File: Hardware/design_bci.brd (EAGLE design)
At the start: 100 x 80 mm, 10 parts, among them IC1 AD623N

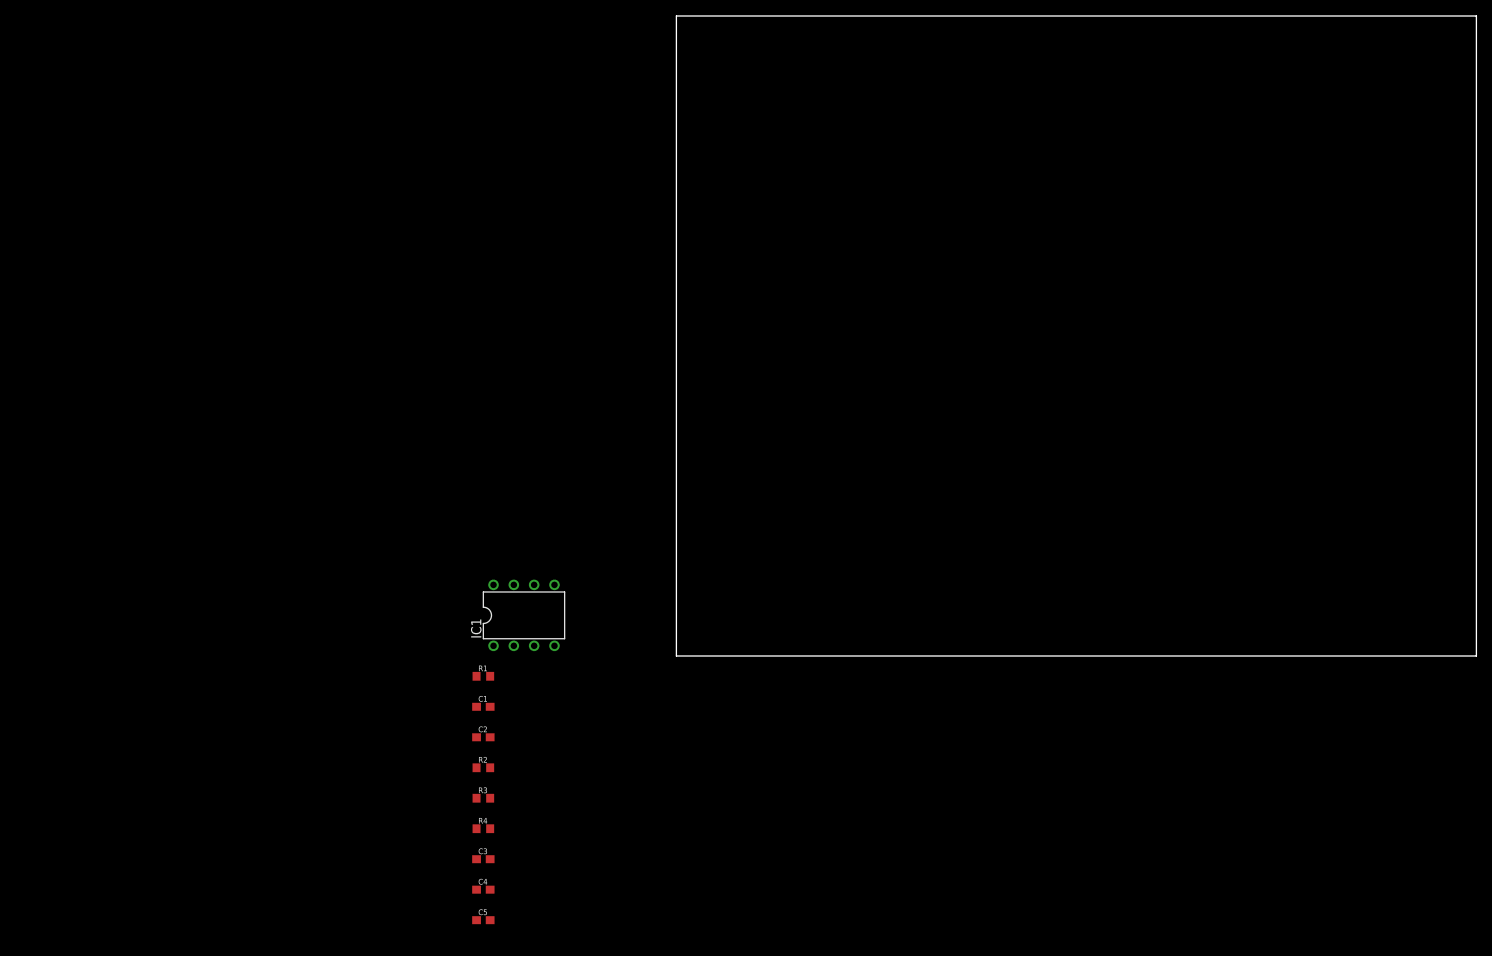
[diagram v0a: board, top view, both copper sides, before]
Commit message: updated
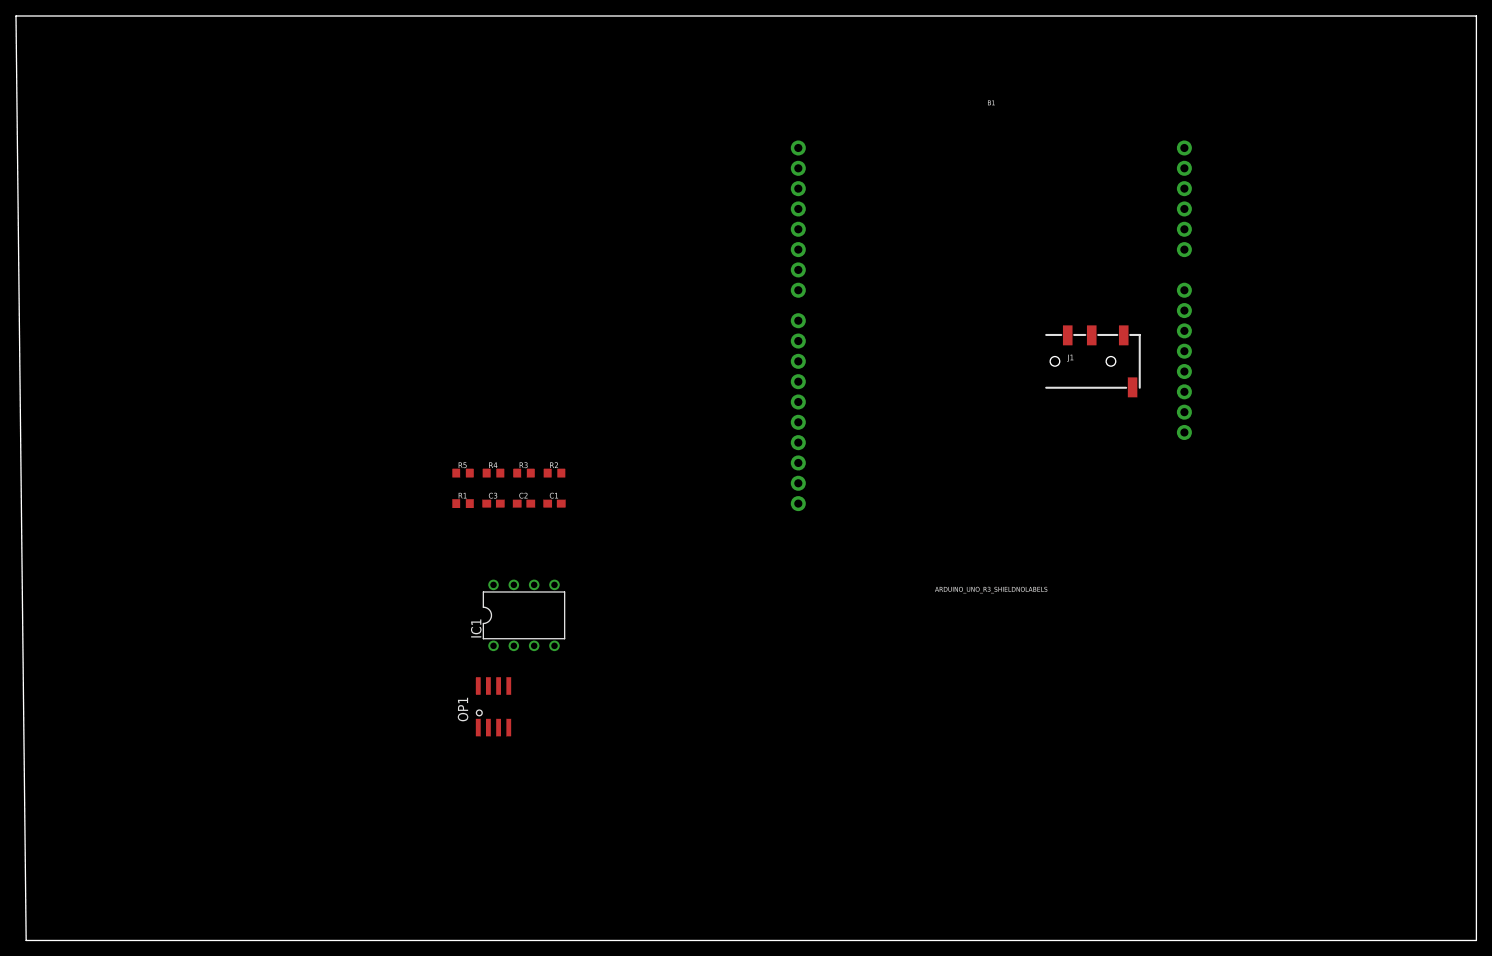
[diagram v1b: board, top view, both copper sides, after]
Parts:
- removed C4, C5: (no value), LinnesLab-Passives:C0603
- added B1: ARDUINO_UNO_R3_SHIELDNOLABELS, LinnesLab-Microcontrollers:UNO_R3_SHIELD_NOLABELS
- added J1: (no value), LinnesLab-Connectors:AUDIO_JACK_3.5MM_TRRS_SMD_RA
- added OP1: (no value), LinnesLab-AnalogIC:SO8
- added R5: (no value), LinnesLab-Passives:R0603
- moved C3 44.5 mm to (-22.9, 19.1)
- moved R4 44.5 mm to (-22.9, 22.9)
- moved R3 41.0 mm to (-19.1, 22.9)
- moved R2 37.9 mm to (-15.2, 22.9)
- moved C2 29.6 mm to (-19.1, 19.1)
- moved C1 26.9 mm to (-15.2, 19.1)
- moved R1 21.7 mm to (-26.7, 19.1)
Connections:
- removed net 5V: C2.1, IC1.7, R3.2
- removed net N$4 (its old number): R3.1, R4.2
- new net 3.3V: C2.1, C3.1, IC1.7, OP1.8, R4.2
- new net N$3: OP1.3, R3.2, R4.1
- new net N$6: IC1.5, OP1.1, OP1.2, OP1.5
- new net N$7: OP1.6, R1.2, R5.1
- new net N$8: OP1.7, R5.2
- net GND: now also C3.2, OP1.4, R3.1; no longer C4.2, R4.1
- net N$1: now also IC1.8, R2.2; no longer IC1.1, R1.2
- net N$2: now also IC1.1, R2.1; no longer IC1.8, R1.1
- net N$5: now also R1.1; no longer R2.1
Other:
- board size 100 x 80 mm -> 182.6 x 115.6 mm
